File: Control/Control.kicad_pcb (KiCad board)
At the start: 2 copper layers, 99 parts, among them J1 Conn_02x04_Odd_Even_Shielded, J2 Conn_01x03, J3 Conn_02x04_Odd_Even_Shielded, J4 Conn_01x03, J5 Conn_02x04_Odd_Even_Shielded, J6 Conn_02x04_Odd_Even_Shielded, J7 Conn_02x04_Odd_Even_Shielded, J8 Conn_02x04_Odd_Even_Shielded, SW1 SW_MEC_5E, SW2 SW_MEC_5E, SW3 SW_MEC_5E, SW4 SW_MEC_5E, SW5 SW_MEC_5E, SW6 SW_MEC_5E

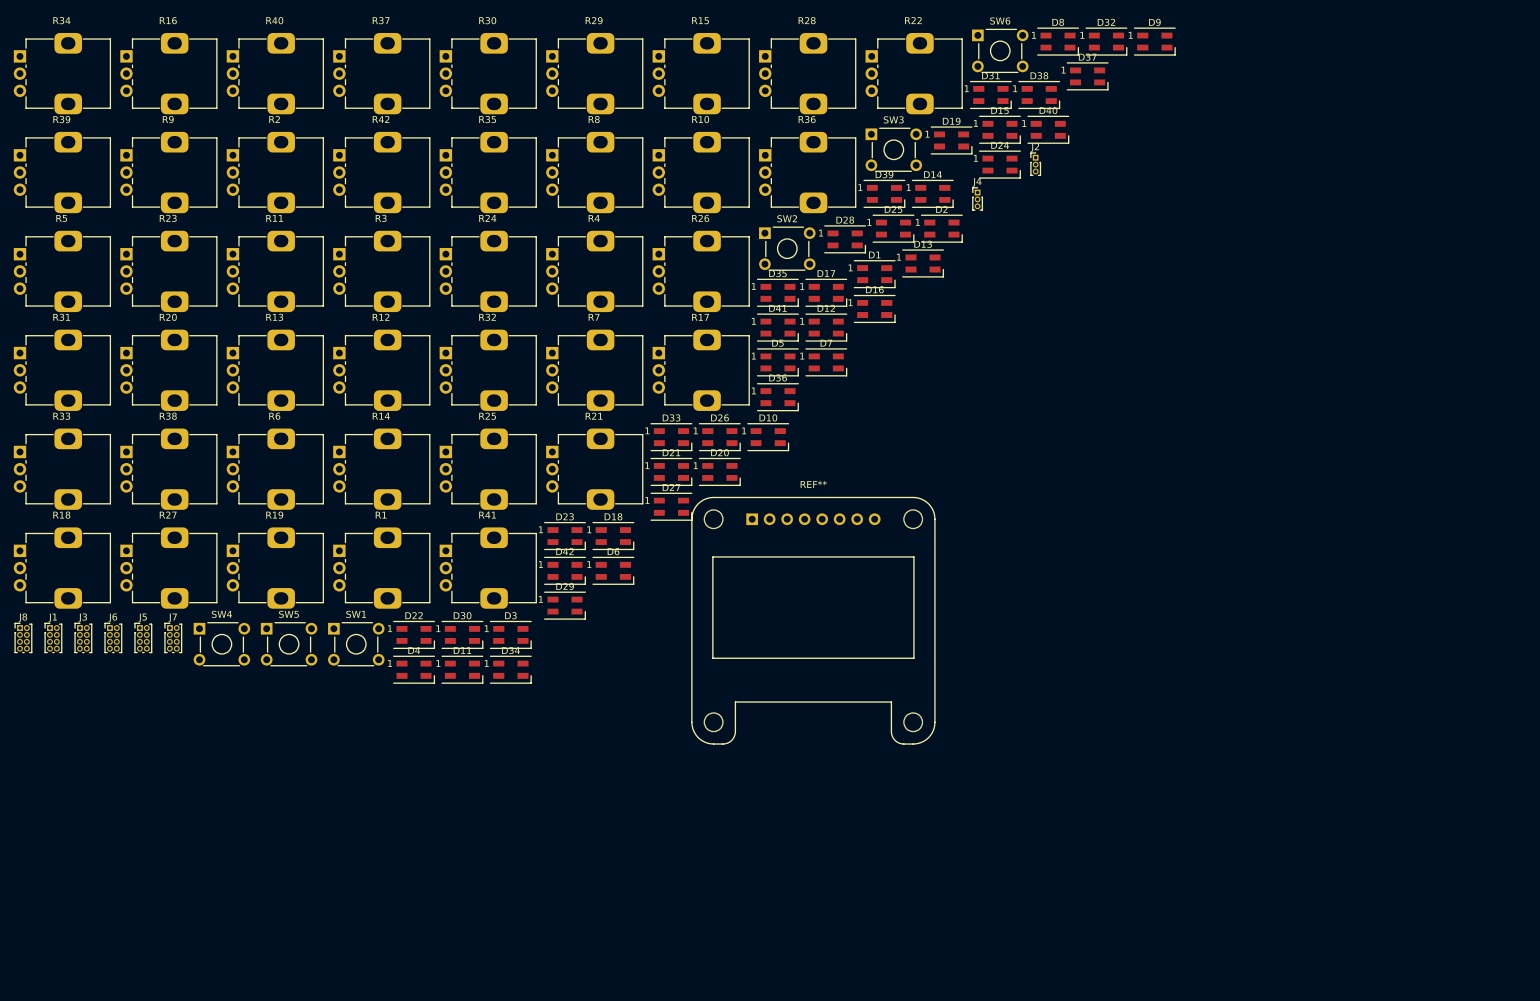
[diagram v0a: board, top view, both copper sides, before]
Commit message: cntrl gerber
easy eda routing
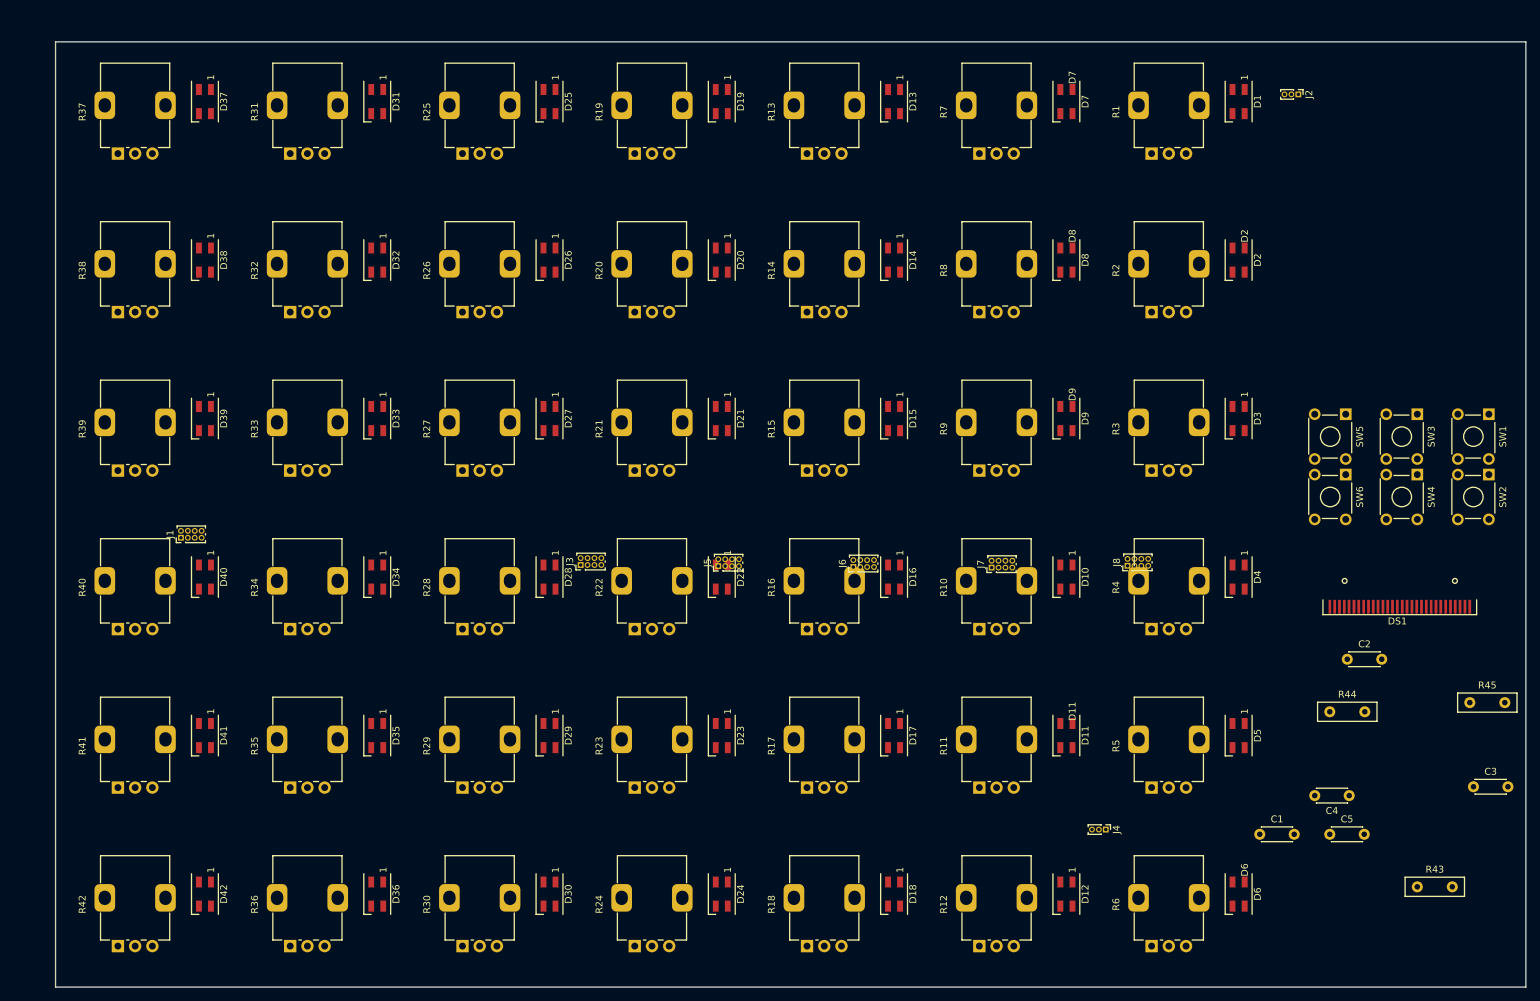
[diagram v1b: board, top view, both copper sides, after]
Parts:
- removed REF**: Adafruit_SSD1306, Display:Adafruit_SSD1306
- added C1: 0.1uF cap, Capacitor_THT:C_Disc_D4.3mm_W1.9mm_P5.00mm, F.Cu at (208.3, 137.2)
- added C2: 4.7uF cap, Capacitor_THT:C_Disc_D4.3mm_W1.9mm_P5.00mm, F.Cu at (221.0, 111.8)
- added C3: 4.7uF/16v, Capacitor_THT:C_Disc_D4.3mm_W1.9mm_P5.00mm, F.Cu at (239.3, 130.3)
- added C4: 0.1uF cap, Capacitor_THT:C_Disc_D4.3mm_W1.9mm_P5.00mm, F.Cu at (221.3, 131.5)
- added C5: 4.7uF/16v, Capacitor_THT:C_Disc_D4.3mm_W1.9mm_P5.00mm, F.Cu at (218.4, 137.2)
- added DS1: OLED-128O064D, Display:OLED-128O064D, F.Cu at (228.6, 104.1)
- added R43: 2.2k, Resistor_THT:R_Box_L8.4mm_W2.5mm_P5.08mm, F.Cu at (231.1, 144.8)
- added R44: 2.2k, Resistor_THT:R_Box_L8.4mm_W2.5mm_P5.08mm, F.Cu at (218.4, 119.4)
- added R45: 560k, Resistor_THT:R_Box_L8.4mm_W2.5mm_P5.08mm, F.Cu at (238.8, 118.0)
- moved R5 181.5 mm to (192.6, 130.4), turned to 90 degrees
- moved SW4 178.1 mm to (231.1, 85.0), turned to -90 degrees
- moved SW1 170.5 mm to (241.5, 76.2), turned to -90 degrees
- moved J8 161.0 mm to (189.1, 98.2), turned to 90 degrees
- moved SW5 159.6 mm to (220.8, 76.2), turned to -90 degrees
- moved R6 151.4 mm to (192.6, 153.4), turned to 90 degrees
- moved D40 138.5 mm to (55.2, 99.8), turned to -90 degrees
- moved R2 135.2 mm to (192.6, 61.4), turned to 90 degrees
- moved R36 133.9 mm to (67.6, 153.4), turned to 90 degrees
- moved R11 133.1 mm to (167.6, 130.4), turned to 90 degrees
- moved R9 131.9 mm to (167.6, 84.4), turned to 90 degrees
- moved R1 131.2 mm to (192.6, 38.4), turned to 90 degrees
- moved R30 129.1 mm to (92.6, 153.4), turned to 90 degrees
- moved R16 129.1 mm to (142.6, 107.4), turned to 90 degrees
- moved D37 128.1 mm to (55.2, 30.8), turned to -90 degrees
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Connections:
- D11 pad 1: Net-(D11-Pad1) -> (no net)
- D11 pad 2: GROUND -> (no net)
- D11 pad 3: 5VDC -> (no net)
- D11 pad 4: Net-(D11-Pad4) -> (no net)
- D2 pad 1: Net-(D2-Pad1) -> (no net)
- D2 pad 2: GROUND -> (no net)
- D2 pad 3: 5VDC -> (no net)
- D2 pad 4: Net-(D2-Pad4) -> (no net)
- D6 pad 1: unconnected-(D6-Pad1) -> (no net)
- D6 pad 2: GROUND -> (no net)
- D6 pad 3: 5VDC -> (no net)
- D6 pad 4: Net-(D12-Pad1) -> (no net)
- D7 pad 1: Net-(D13-Pad4) -> (no net)
- D7 pad 2: GROUND -> (no net)
- D7 pad 3: 5VDC -> (no net)
- D7 pad 4: Net-(D1-Pad1) -> (no net)
- D8 pad 1: Net-(D14-Pad4) -> (no net)
- D8 pad 2: GROUND -> (no net)
- D8 pad 3: 5VDC -> (no net)
- D8 pad 4: Net-(D2-Pad1) -> (no net)
- D9 pad 1: Net-(D15-Pad4) -> (no net)
- D9 pad 2: GROUND -> (no net)
- D9 pad 3: 5VDC -> (no net)
- D9 pad 4: Net-(D3-Pad1) -> (no net)
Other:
- board outline added: 213.4 x 137.2 mm
